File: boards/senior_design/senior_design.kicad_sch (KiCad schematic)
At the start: 10 parts

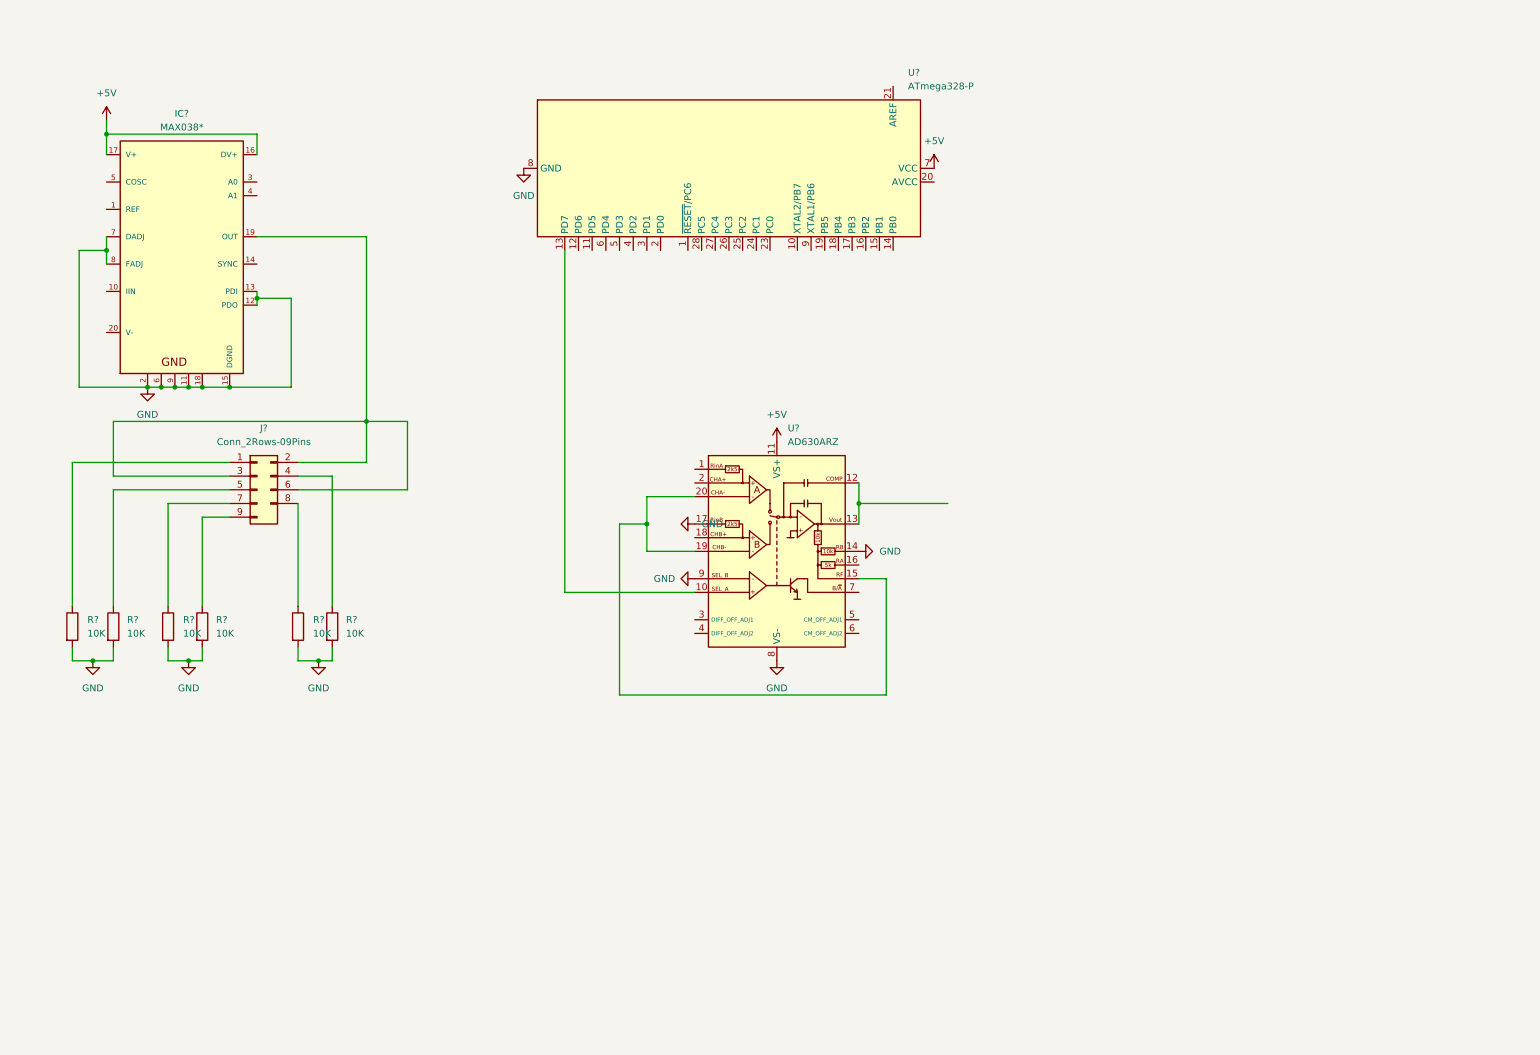
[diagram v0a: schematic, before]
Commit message: finished schematic
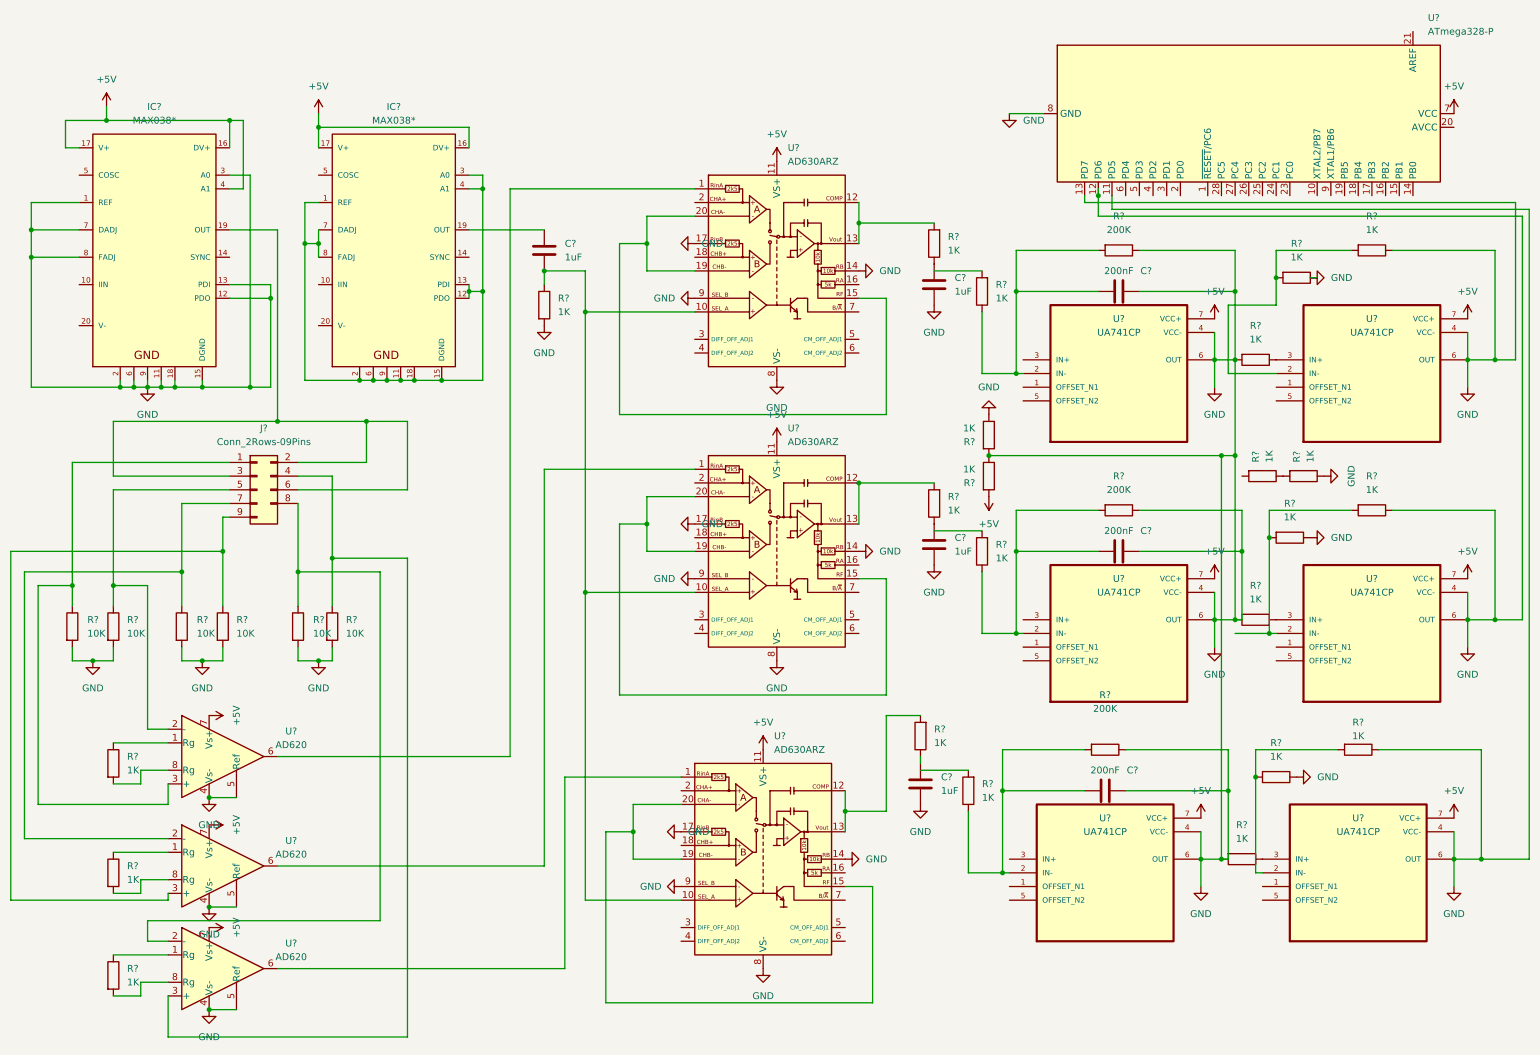
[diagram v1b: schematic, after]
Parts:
- added C? (x4): 1uF, symbol Device:C
- added C? (x3): 200nF, symbol Device:C
- added IC?: MAX038*, symbol MAX038_:MAX038*
- added R? (x23): 1K, symbol Device:R
- added R? (x3): 200K, symbol Device:R
- added U? (x6): UA741CP, DIP794W45P254L959H508Q8, symbol uA741:UA741CP
- added U? (x3): AD620, symbol Amplifier_Instrumentation:AD620
- added U? (x2): AD630ARZ, Package_SO:SOIC-20W_7.5x12.8mm_P1.27mm, symbol Analog:AD630ARZ
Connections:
- net +5V: now also IC?.4 (A1), IC?.16 (DV+), IC?.17 (V+), R?.2, U?.11 (VS+), U?.11 (VS+), U?.7 (VCC+), U?.7 (VCC+), U?.7 (VCC+), U?.7 (VCC+), U?.7 (VCC+), U?.7 (VCC+), U?.7 (Vs+), U?.7 (Vs+), U?.7 (Vs+)
- net GND: now also IC?.1 (REF), IC?.3 (A0), U?.11 (PD5), U?.12 (PD6), U?.13 (PD7), C?.1, C?.1, C?.1, C?.1, C?.1, C?.1, R?.1, R?.1, R?.1, R?.1, R?.1, R?.1, R?.1, R?.1, R?.1, R?.1, R?.1, R?.1, R?.2, R?.2, R?.2, R?.2, R?.2, U?.14 (RB), U?.14 (RB), U?.17 (RinB), U?.17 (RinB), U?.4 (VCC-), U?.4 (VCC-), U?.4 (VCC-), U?.4 (VCC-), U?.4 (VCC-), U?.4 (VCC-), U?.4 (Vs-), U?.4 (Vs-), U?.4 (Vs-), U?.5 (Ref), U?.5 (Ref), U?.5 (Ref), U?.6 (OUT), U?.6 (OUT), U?.6 (OUT), U?.6 (OUT), U?.6 (OUT), U?.6 (OUT), U?.8 (VS-), U?.8 (VS-), U?.9 (SEL_B), U?.9 (SEL_B)
- net at U?.10 (SEL_A): now also C?.2, R?.1, U?.10 (SEL_A), U?.10 (SEL_A); no longer U?.13 (PD7)
- net at J?.7 (Pin_7), R?.1: now also U?.2 (-)
- net at U?.1 (RinA): now also U?.6
- net at U?.12 (COMP), U?.13 (Vout): now also R?.2
- net at J?.9 (Pin_9), R?.1: now also U?.3 (+)
- net at J?.1 (Pin_1), R?.1: now also U?.3 (+)
- net at J?.4 (Pin_4), R?.1: now also U?.3 (+)
- net at J?.5 (Pin_5), R?.1: now also U?.2 (-)
- net at J?.8 (Pin_8), R?.1: now also U?.2 (-)
- new net: R?.1, U?.3 (IN+) (x3)
- new net: C?.2, R?.1 (x3)
- new net: C?.2, R?.1, R?.2, U?.2 (IN-) (x3)
- new net: R?.1, U?.1 (Rg) (x3)
- new net: R?.2, U?.8 (Rg) (x3)
- new net: R?.2, U?.12 (COMP), U?.13 (Vout) (x2)
- new net: R?.2, R?.2, U?.2 (IN-) (x3)
- new net: R?.1, R?.2
- new net: U?.1 (RinA), U?.6 (x2)
- new net: U?.15 (RF), U?.19 (CHB-), U?.20 (CHA-) (x2)
- new net: IC?.1 (REF), IC?.11, IC?.12 (PDO), IC?.13 (PDI), IC?.15 (DGND), IC?.18, IC?.2, IC?.3 (A0), IC?.4 (A1), IC?.6, IC?.7 (DADJ), IC?.8 (FADJ), IC?.9
- new net: C?.1, IC?.19 (OUT)
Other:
- moved on the sheet: IC?, R?, U?
